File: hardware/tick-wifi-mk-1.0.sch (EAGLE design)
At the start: 35 parts, among them IC1 MAX7219, IC2 MAX7219, IC3 74HC125, IC4 LD1117 5V, IC5 LD1117 3V, Q1 MMBT2222, Q2 MMBT2222

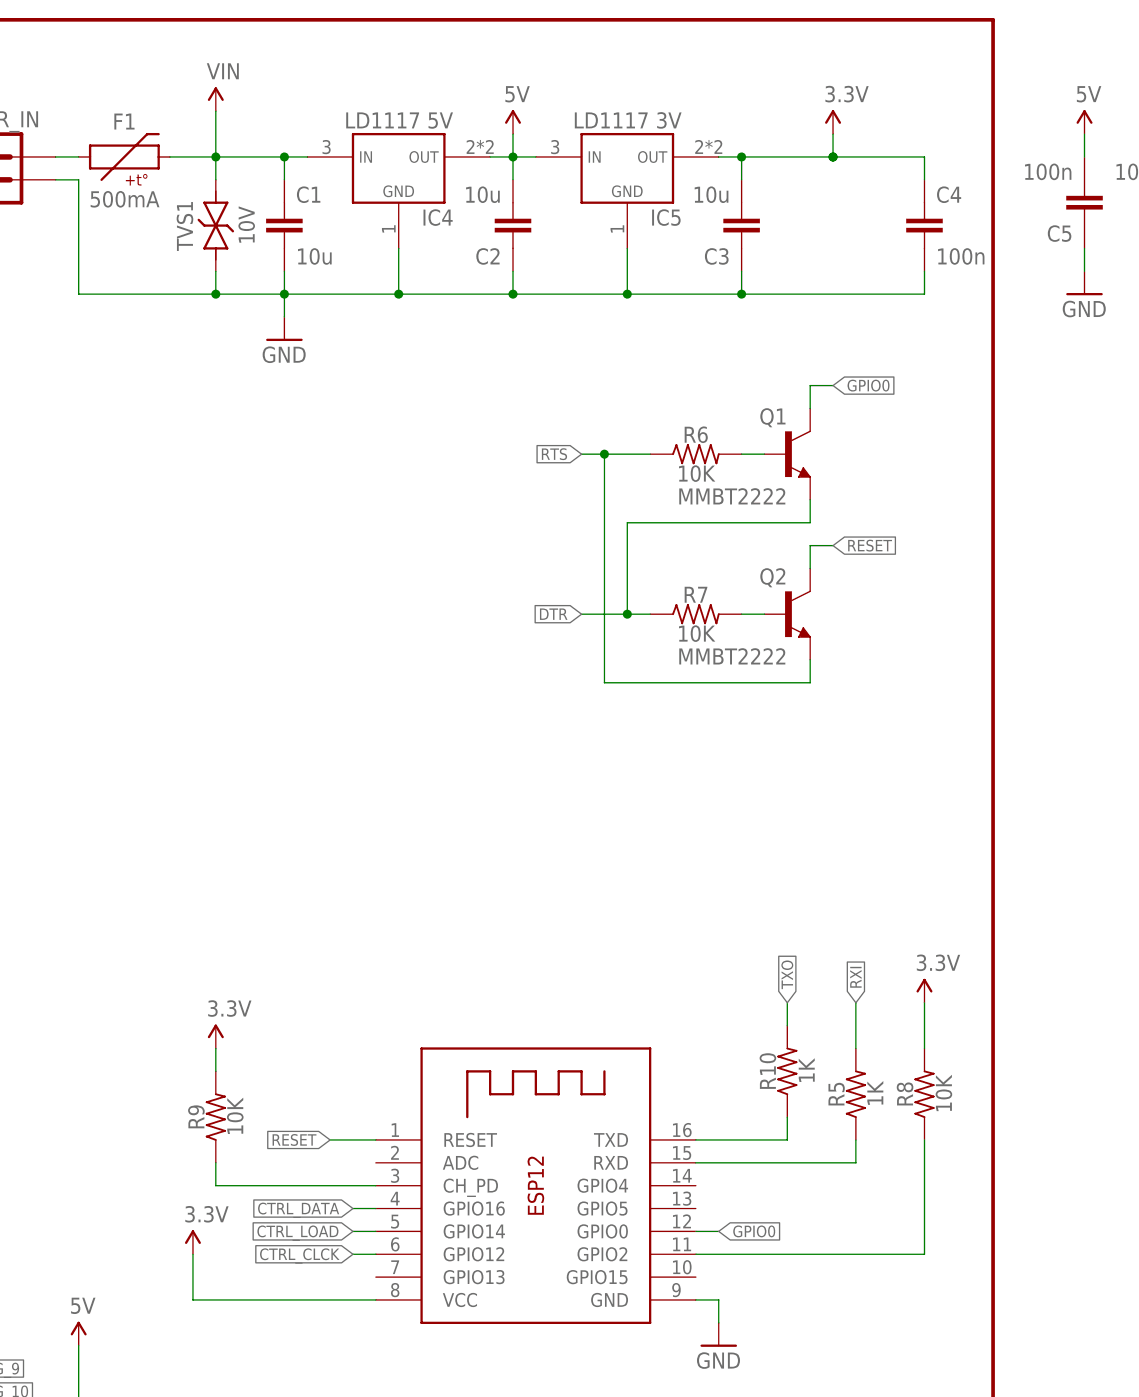
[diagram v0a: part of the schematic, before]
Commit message: wip
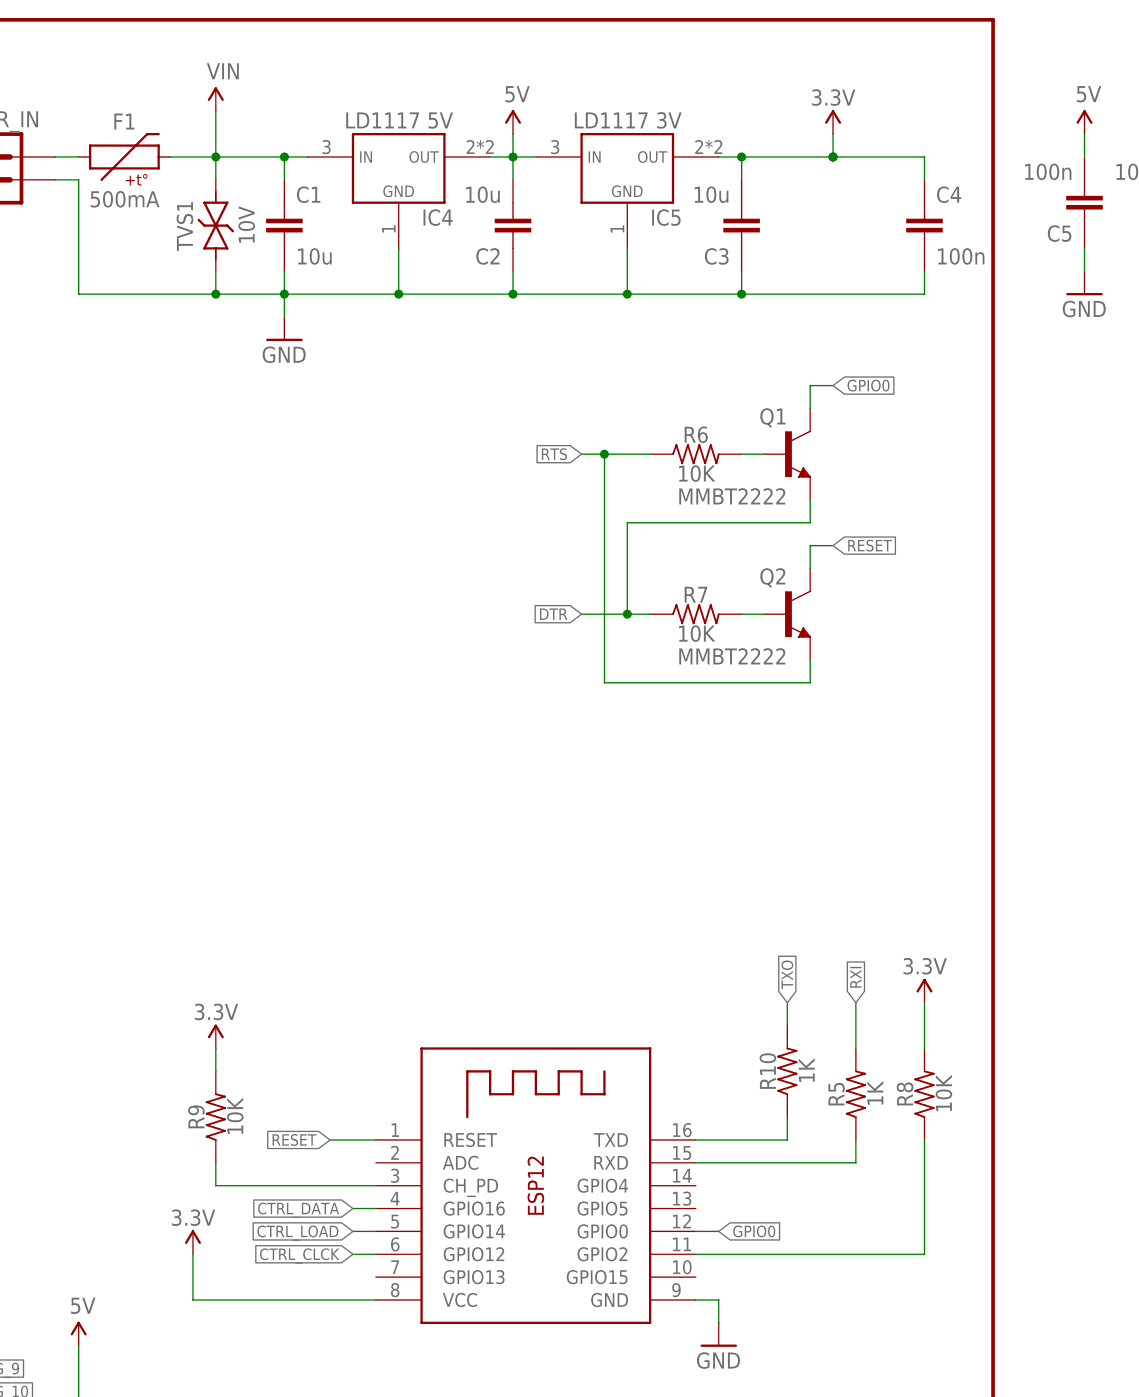
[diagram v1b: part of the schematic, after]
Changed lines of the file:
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@@
 <?xml version="1.0" encoding="utf-8"?>
 <!DOCTYPE eagle SYSTEM "eagle.dtd">
-<eagle version="6.5.0">
+<eagle version="7.5.0">
 <drawing>
 <settings>

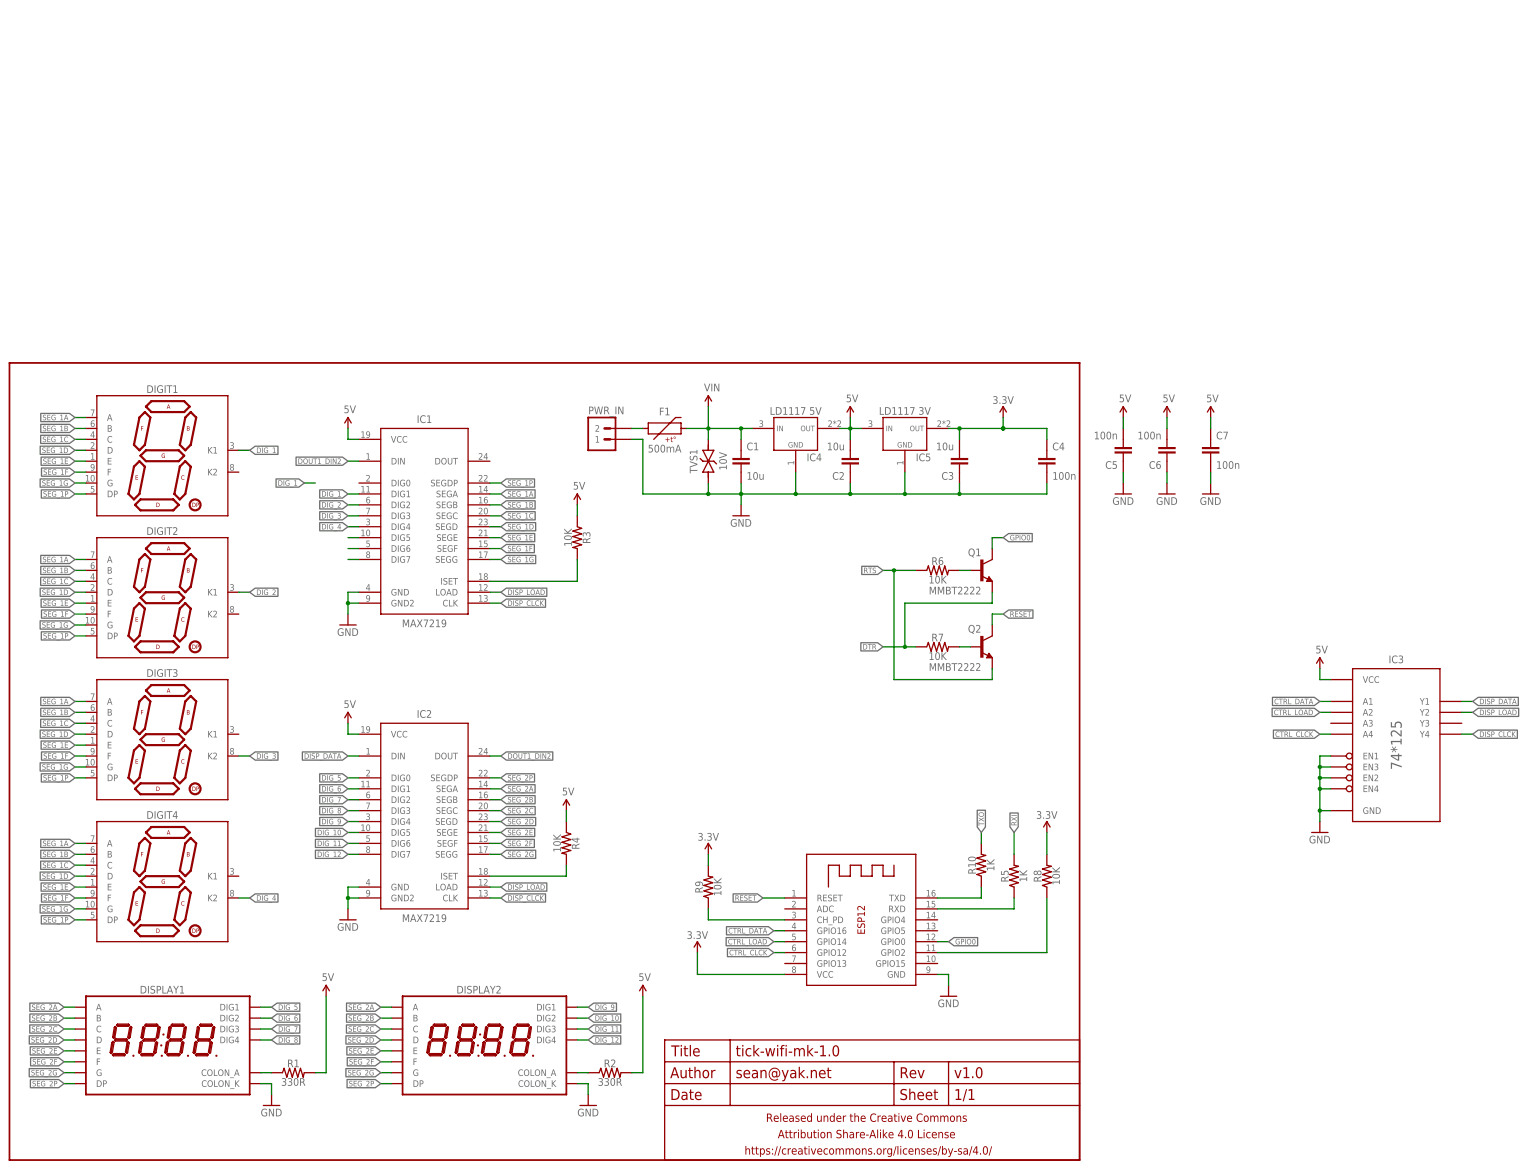
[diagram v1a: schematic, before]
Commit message: more wip
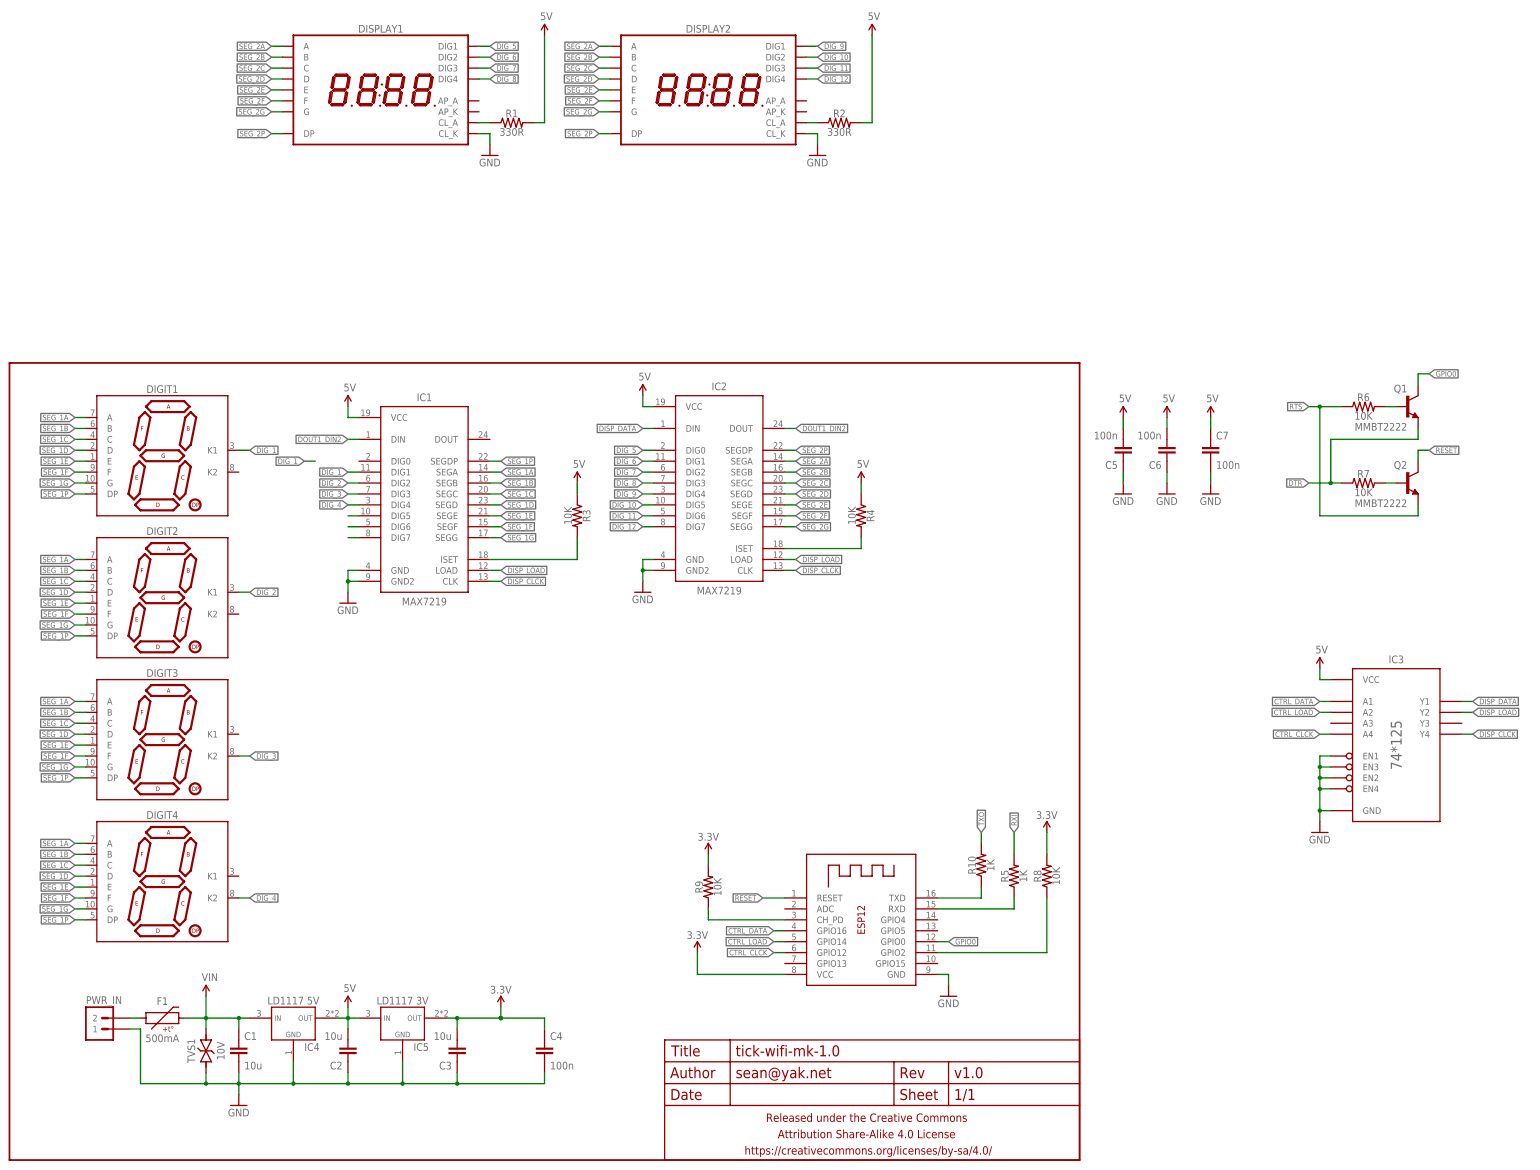
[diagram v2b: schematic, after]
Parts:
- DIGIT1, DIGIT2, DIGIT3, DIGIT4: device A_butts:7SEG_1DIGPTH-25.4MM-BARE -> a_parts:7SEG_1DIGPTH-25.4MM-BARE
- DISPLAY1, DISPLAY2: value 7SEG_4DIGIT_COLON14.2MM-CC -> 7SEG_4DIGIT_COLON_APOS; device a_parts:7SEG_4DIGIT_COLON14.2MM-CC -> a_parts:7SEG_4DIGIT_COLON_APOS
- F1: device A_butts:PTCPTC-1210 -> a_parts:PTCPTC-1210
- FRAME1: device A_butts:FRAME-LETTERNO_PACKAGE -> a_parts:FRAME-LETTERNO_PACKAGE
- PWR_IN: device A_butts:M02PTH-CENTERED-R+ -> a_parts:M02PTH-CENTERED-R+
- TVS1: device A_butts:TVSSMA -> a_parts:TVSSMA
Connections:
- net GND: now also DISPLAY1.CL_K, DISPLAY2.CL_K; no longer DISPLAY1.COLON_K, DISPLAY2.COLON_K
- net N$3: now also DISPLAY1.CL_A; no longer DISPLAY1.COLON_A
- net N$5: now also DISPLAY2.CL_A; no longer DISPLAY2.COLON_A
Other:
- moved on the sheet: C1, C2, C3, C4, F1, IC1, IC2, IC4, IC5, PWR_IN, Q1, Q2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
